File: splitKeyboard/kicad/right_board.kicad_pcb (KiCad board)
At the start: 2 copper layers, 305 x 136.1 mm, 131 parts

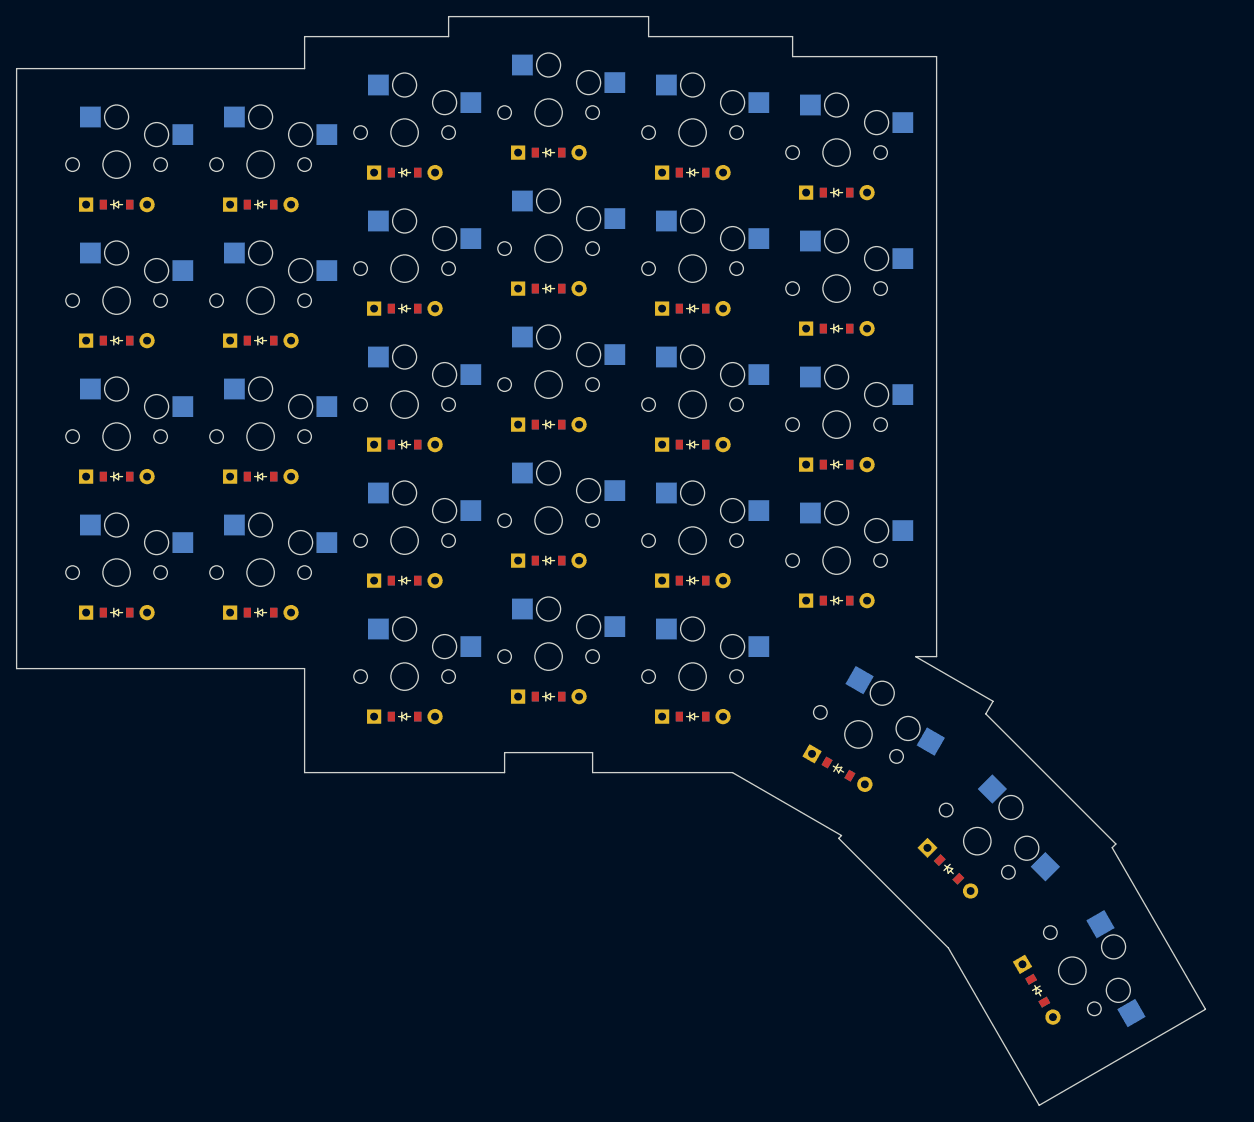
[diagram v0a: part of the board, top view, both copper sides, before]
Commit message: fix: got rid of unnecessary extra side
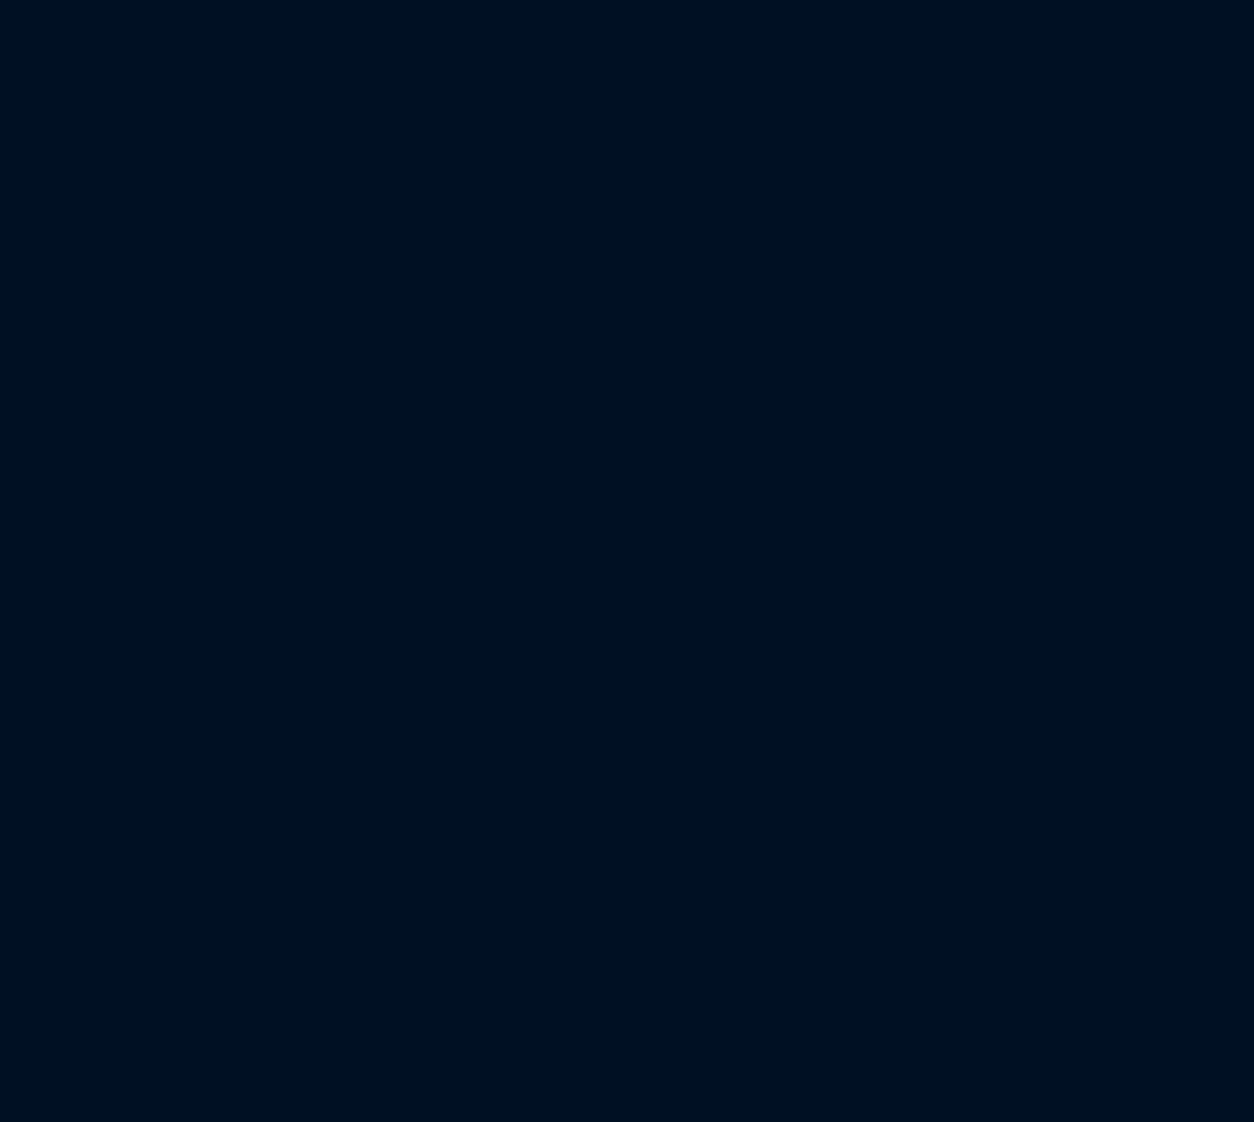
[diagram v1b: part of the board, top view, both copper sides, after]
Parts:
- removed D33, D34, D35, D36, D37, D38, D39, D40, D41, D42, D43, D44, D45, D46, D47, D48, D49, D50, D51, D52, D53, D54, D55, D56, D57, D58, D59, D60, D61, D62: , ComboDiode
- removed S31, S32, S33, S34, S35, S36, S37, S38, S39, S40, S41, S42, S43, S44, S45, S46, S47, S48, S49, S50, S51, S52, S53, S54, S55, S56, S57, S58, S59, S60: , PG1350
- moved D1 280.0 mm to (380.0, 88.0)
- moved D2 280.0 mm to (380.0, 71.0)
- moved D3 280.0 mm to (380.0, 54.0)
- moved D4 280.0 mm to (380.0, 37.0)
- moved S1 280.0 mm to (380.0, 83.0)
- moved S2 280.0 mm to (380.0, 66.0)
- moved S3 280.0 mm to (380.0, 49.0)
- moved S4 280.0 mm to (380.0, 32.0)
- moved D5 244.0 mm to (362.0, 88.0)
- moved D6 244.0 mm to (362.0, 71.0)
- moved D7 244.0 mm to (362.0, 54.0)
- moved D8 244.0 mm to (362.0, 37.0)
- moved S5 244.0 mm to (362.0, 83.0)
- moved S6 244.0 mm to (362.0, 66.0)
- moved S7 244.0 mm to (362.0, 49.0)
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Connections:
- D1 pad 2: outer_bottom -> mirror_outer_bottom
- D10 pad 2: ring_bottom -> mirror_ring_bottom
- D11 pad 2: ring_home -> mirror_ring_home
- D12 pad 2: ring_top -> mirror_ring_top
- D13 pad 2: ring_num -> mirror_ring_num
- D14 pad 2: middle_mod -> mirror_middle_mod
- D15 pad 2: middle_bottom -> mirror_middle_bottom
- D16 pad 2: middle_home -> mirror_middle_home
- D17 pad 2: middle_top -> mirror_middle_top
- D18 pad 2: middle_num -> mirror_middle_num
- D19 pad 2: index_mod -> mirror_index_mod
- D2 pad 2: outer_home -> mirror_outer_home
- D20 pad 2: index_bottom -> mirror_index_bottom
- D21 pad 2: index_home -> mirror_index_home
- D22 pad 2: index_top -> mirror_index_top
- D23 pad 2: index_num -> mirror_index_num
- D24 pad 2: inner_bottom -> mirror_inner_bottom
- D25 pad 2: inner_home -> mirror_inner_home
- D26 pad 2: inner_top -> mirror_inner_top
- D27 pad 2: inner_num -> mirror_inner_num
- D28 pad 2: layer_cluster -> mirror_layer_cluster
- D29 pad 2: space_cluster -> mirror_space_cluster
- D3 pad 2: outer_top -> mirror_outer_top
- D30 pad 2: extra_cluster -> mirror_extra_cluster
- D31 pad 1: P7 -> GND
- D31 pad 2: mirror_outer_bottom -> P0
- D32 pad 1: P6 -> GND
- D32 pad 2: mirror_outer_home -> VCC
- D4 pad 2: outer_num -> mirror_outer_num
- D5 pad 2: pinky_bottom -> mirror_pinky_bottom
- D6 pad 2: pinky_home -> mirror_pinky_home
- D7 pad 2: pinky_top -> mirror_pinky_top
- D8 pad 2: pinky_num -> mirror_pinky_num
- D9 pad 2: ring_mod -> mirror_ring_mod
- S1 pad 2: outer_bottom -> mirror_outer_bottom
- S10 pad 2: ring_bottom -> mirror_ring_bottom
- S11 pad 2: ring_home -> mirror_ring_home
- S12 pad 2: ring_top -> mirror_ring_top
- S13 pad 2: ring_num -> mirror_ring_num
- S14 pad 2: middle_mod -> mirror_middle_mod
- S15 pad 2: middle_bottom -> mirror_middle_bottom
- S16 pad 2: middle_home -> mirror_middle_home
- S17 pad 2: middle_top -> mirror_middle_top
- S18 pad 2: middle_num -> mirror_middle_num
- S19 pad 2: index_mod -> mirror_index_mod
- S2 pad 2: outer_home -> mirror_outer_home
- S20 pad 2: index_bottom -> mirror_index_bottom
- S21 pad 2: index_home -> mirror_index_home
- S22 pad 2: index_top -> mirror_index_top
- S23 pad 2: index_num -> mirror_index_num
- S24 pad 2: inner_bottom -> mirror_inner_bottom
- S25 pad 2: inner_home -> mirror_inner_home
- S26 pad 2: inner_top -> mirror_inner_top
- S27 pad 2: inner_num -> mirror_inner_num
- S28 pad 2: layer_cluster -> mirror_layer_cluster
- S29 pad 2: space_cluster -> mirror_space_cluster
- S3 pad 2: outer_top -> mirror_outer_top
- S30 pad 2: extra_cluster -> mirror_extra_cluster
- S4 pad 2: outer_num -> mirror_outer_num
- S5 pad 2: pinky_bottom -> mirror_pinky_bottom
- S6 pad 2: pinky_home -> mirror_pinky_home
- S7 pad 2: pinky_top -> mirror_pinky_top
- S8 pad 2: pinky_num -> mirror_pinky_num
- S9 pad 2: ring_mod -> mirror_ring_mod
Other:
- board size 305 x 136.1 mm -> 148.6 x 136.1 mm

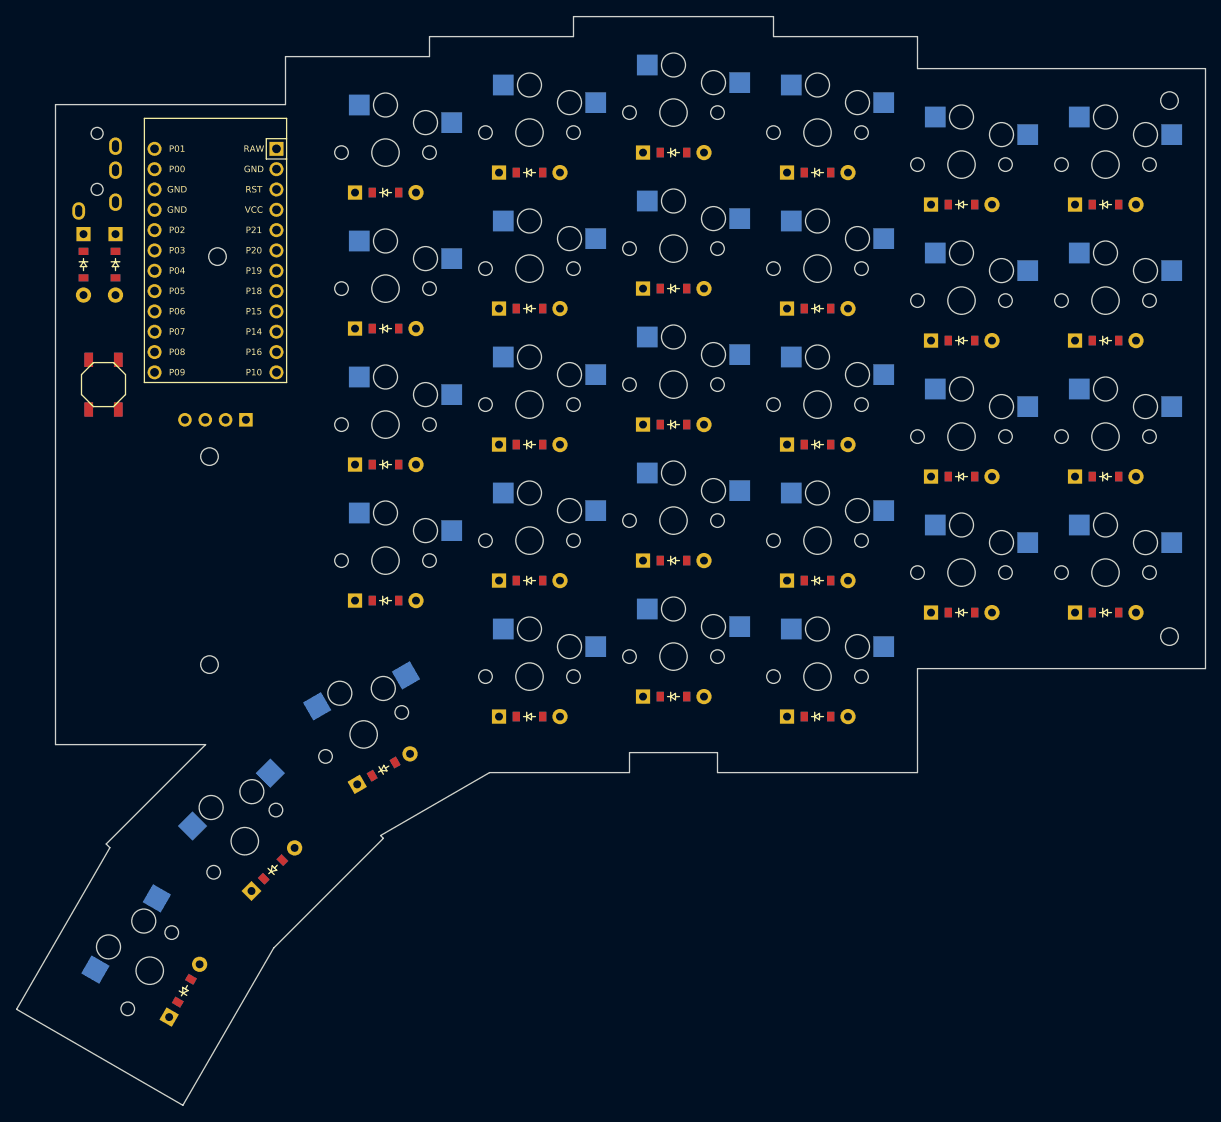
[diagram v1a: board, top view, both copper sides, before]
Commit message: feat(right_board): right board traced
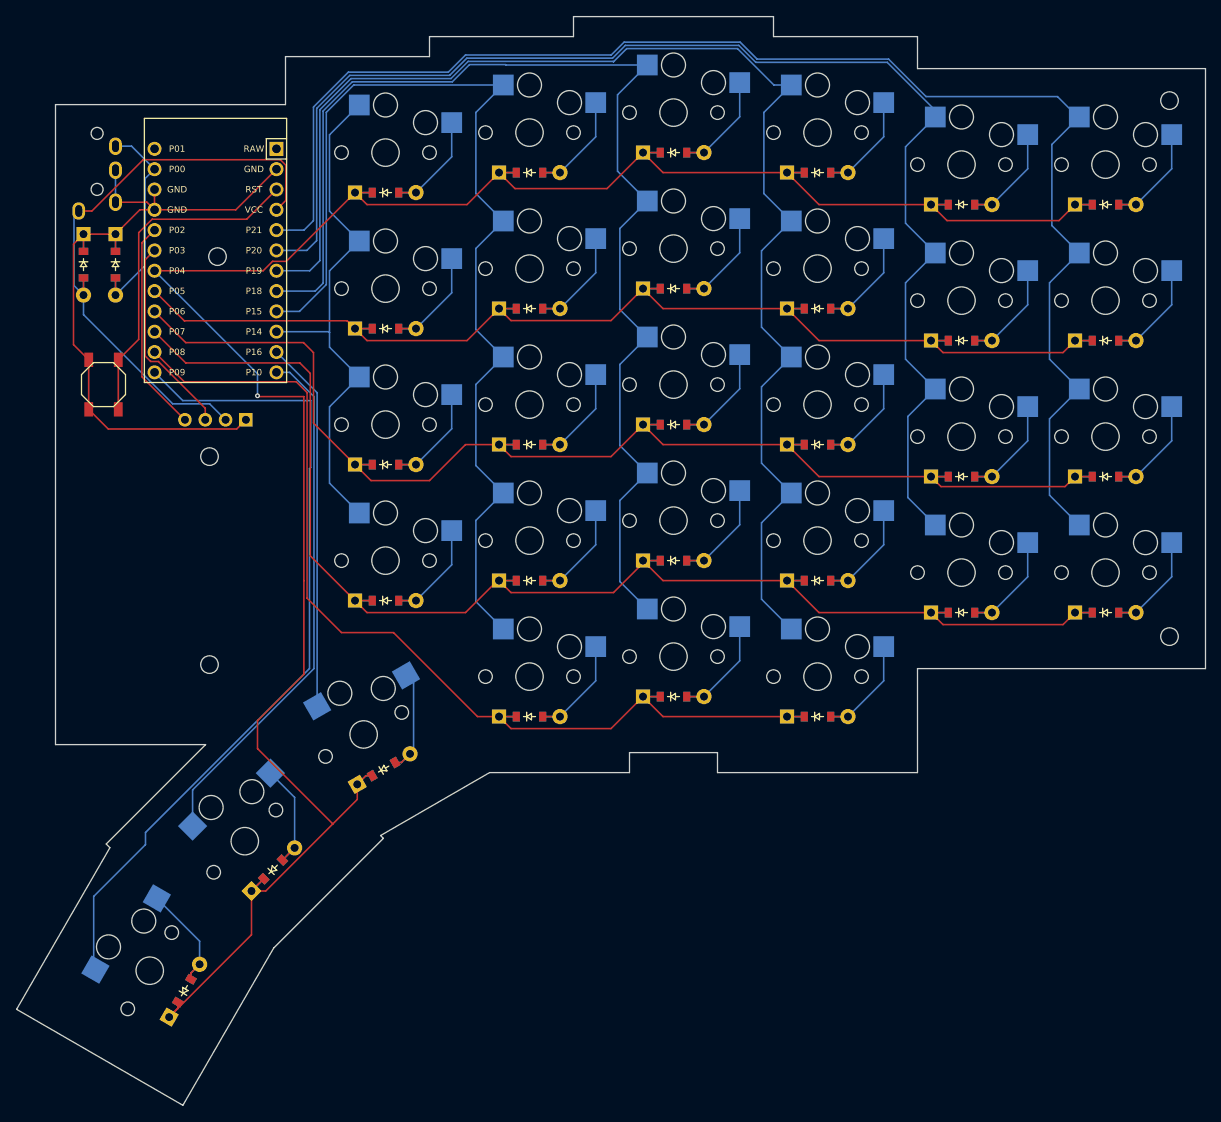
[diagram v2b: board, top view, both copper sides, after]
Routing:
- net P4: track 0.00 -> 294.3 mm, vias 0 -> 1
- net P21: track 0.00 -> 182.3 mm
- net P7: track 0.00 -> 176.9 mm
- net P19: track 0.00 -> 168.9 mm
- net P20: track 0.00 -> 166.9 mm
- net P6: track 0.00 -> 162.8 mm
- net P5: track 0.00 -> 151.4 mm
- net P18: track 0.00 -> 150.3 mm
- net P15: track 0.00 -> 132.0 mm
- net P8: track 0.00 -> 129.3 mm
- net P9: track 0.00 -> 103.4 mm
- net GND: track 0.00 -> 92.3 mm
- net VCC: track 0.00 -> 76.1 mm
- net P14: track 0.00 -> 66.9 mm
- net P10: track 0.00 -> 65.9 mm
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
